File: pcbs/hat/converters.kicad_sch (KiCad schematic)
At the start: 10 parts, among them U18 ADS7828, U19 ADS7828, U20 ADS7828, U21 ???

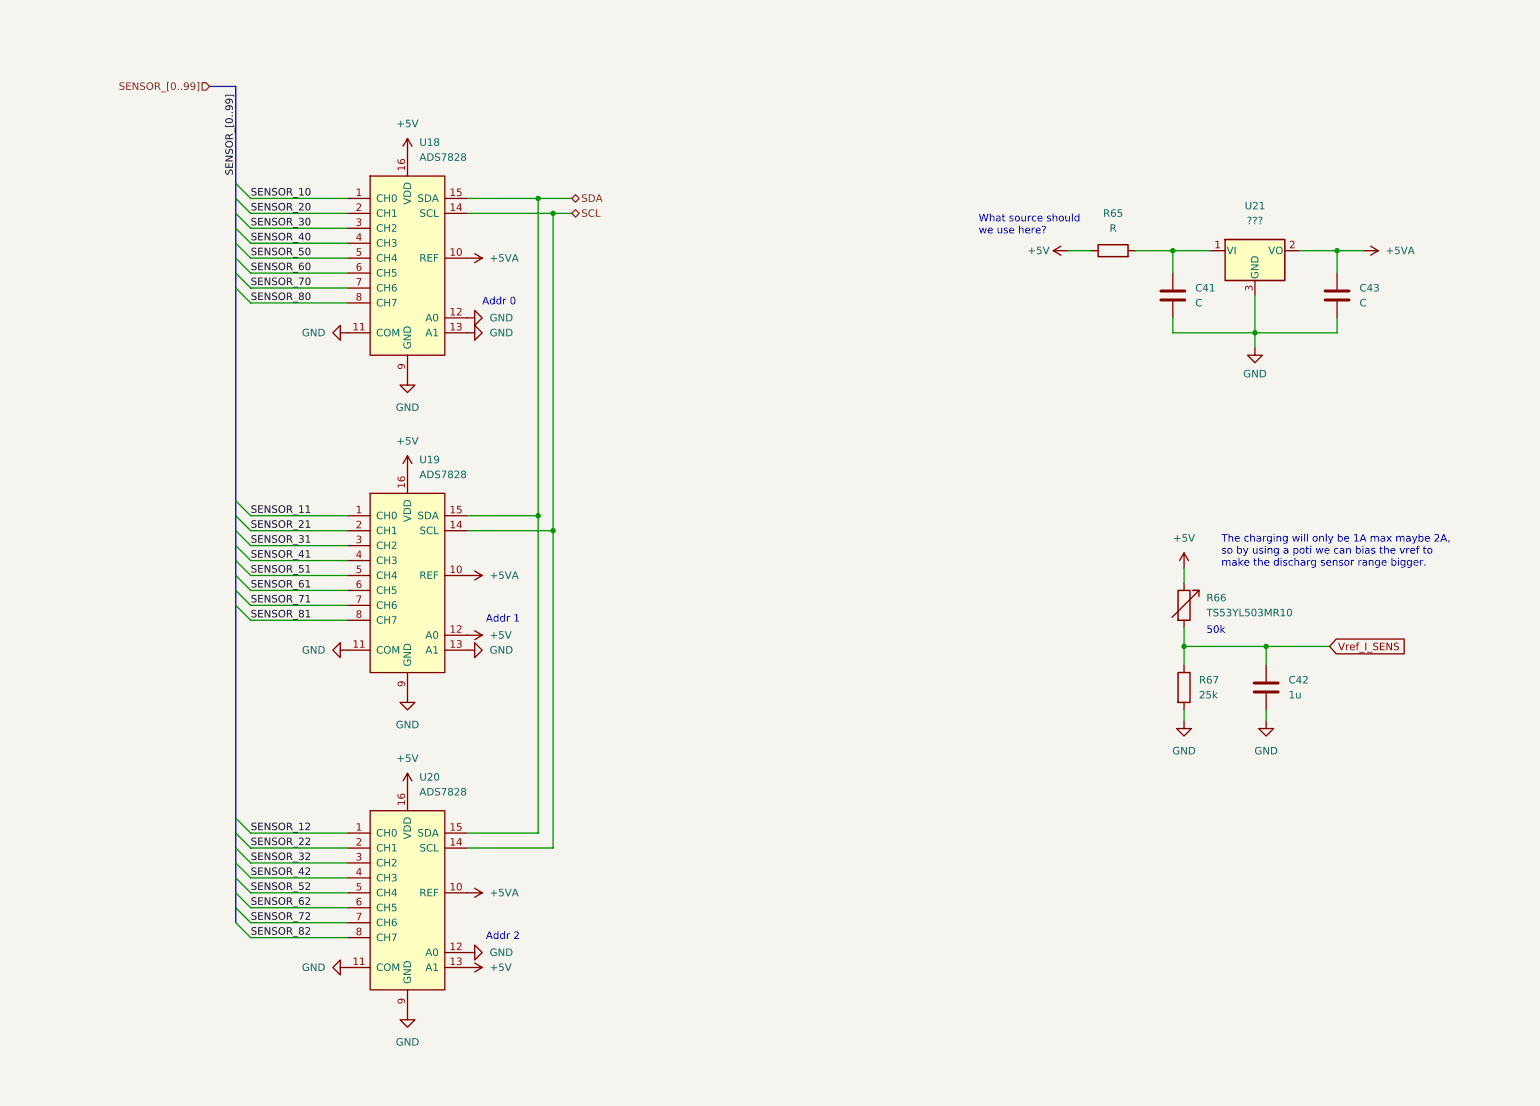
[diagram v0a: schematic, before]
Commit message: formatting
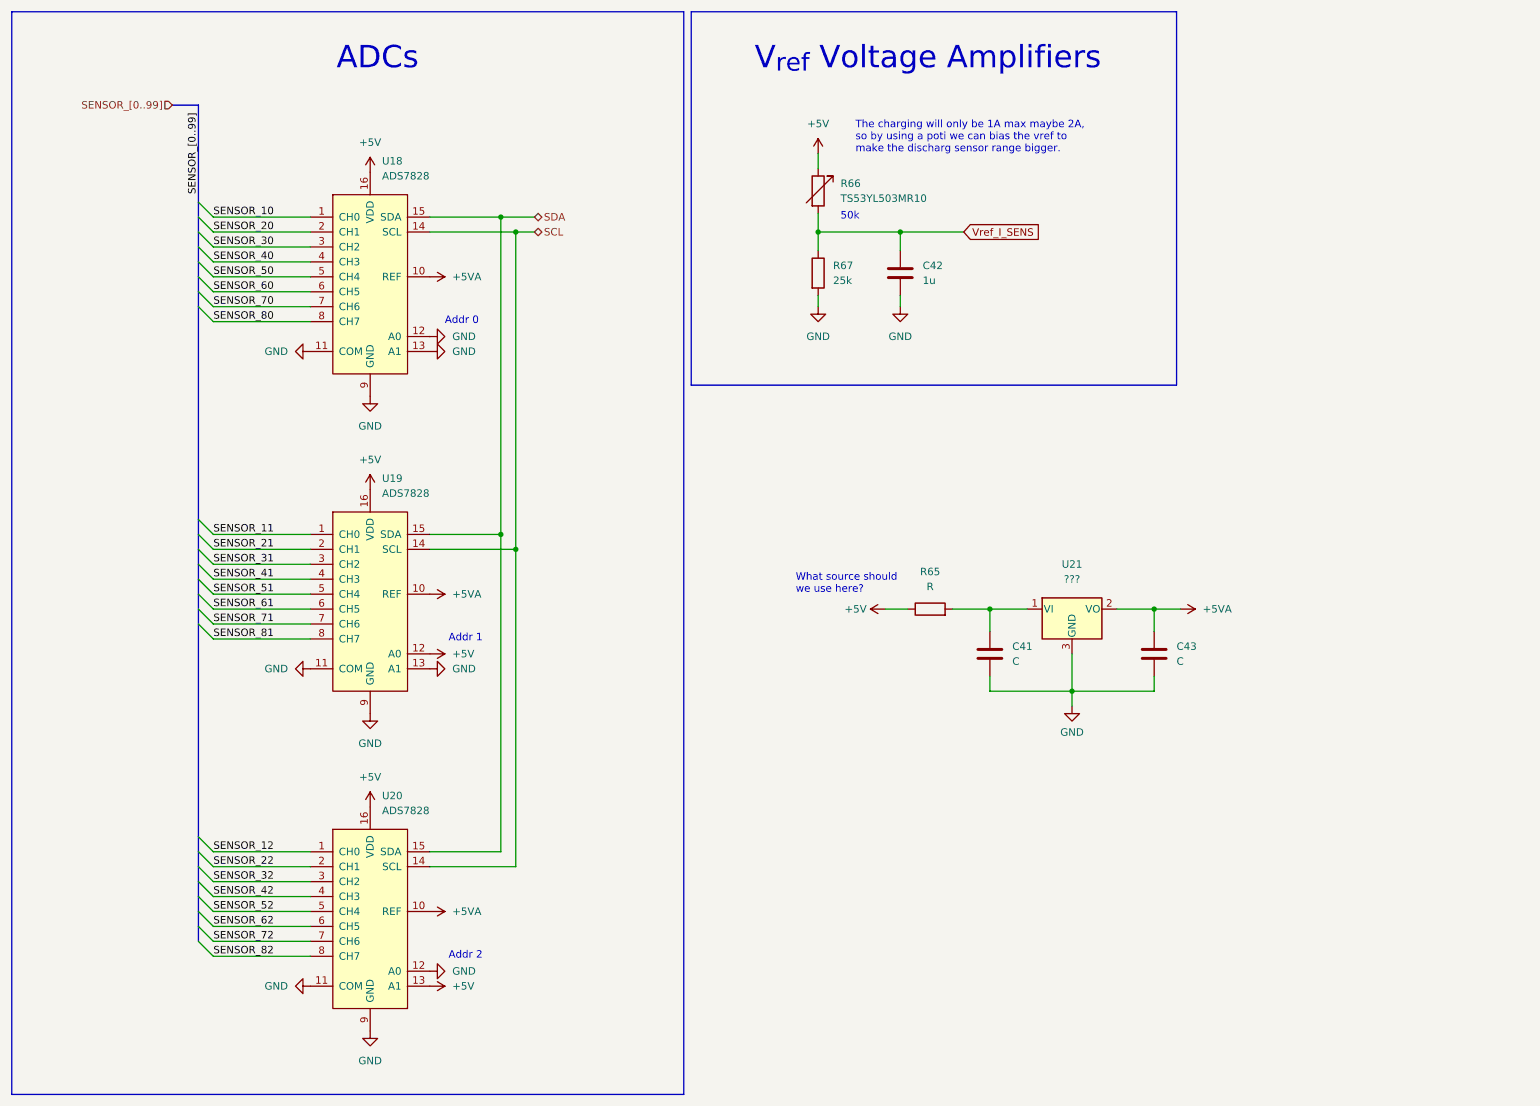
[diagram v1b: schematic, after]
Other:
- note added: "ADCs"
- note added: "V_{ref} Voltage Amplifiers"
- moved on the sheet: C41, C42, C43, R65, R66, R67, U18, U19, U20, U21
